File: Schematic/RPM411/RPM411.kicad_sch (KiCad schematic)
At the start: 84 parts, among them J1 02x08_tbd, P1 P_Cap, Q1 tbd (GDS), U1 STM32F100C8Tb8, U2 TS5A9411, U3 TS5A9411, U4 TS5A9411, U5 74LVC3G04, U6 74LVC1G32, U7 TLV70030DDC

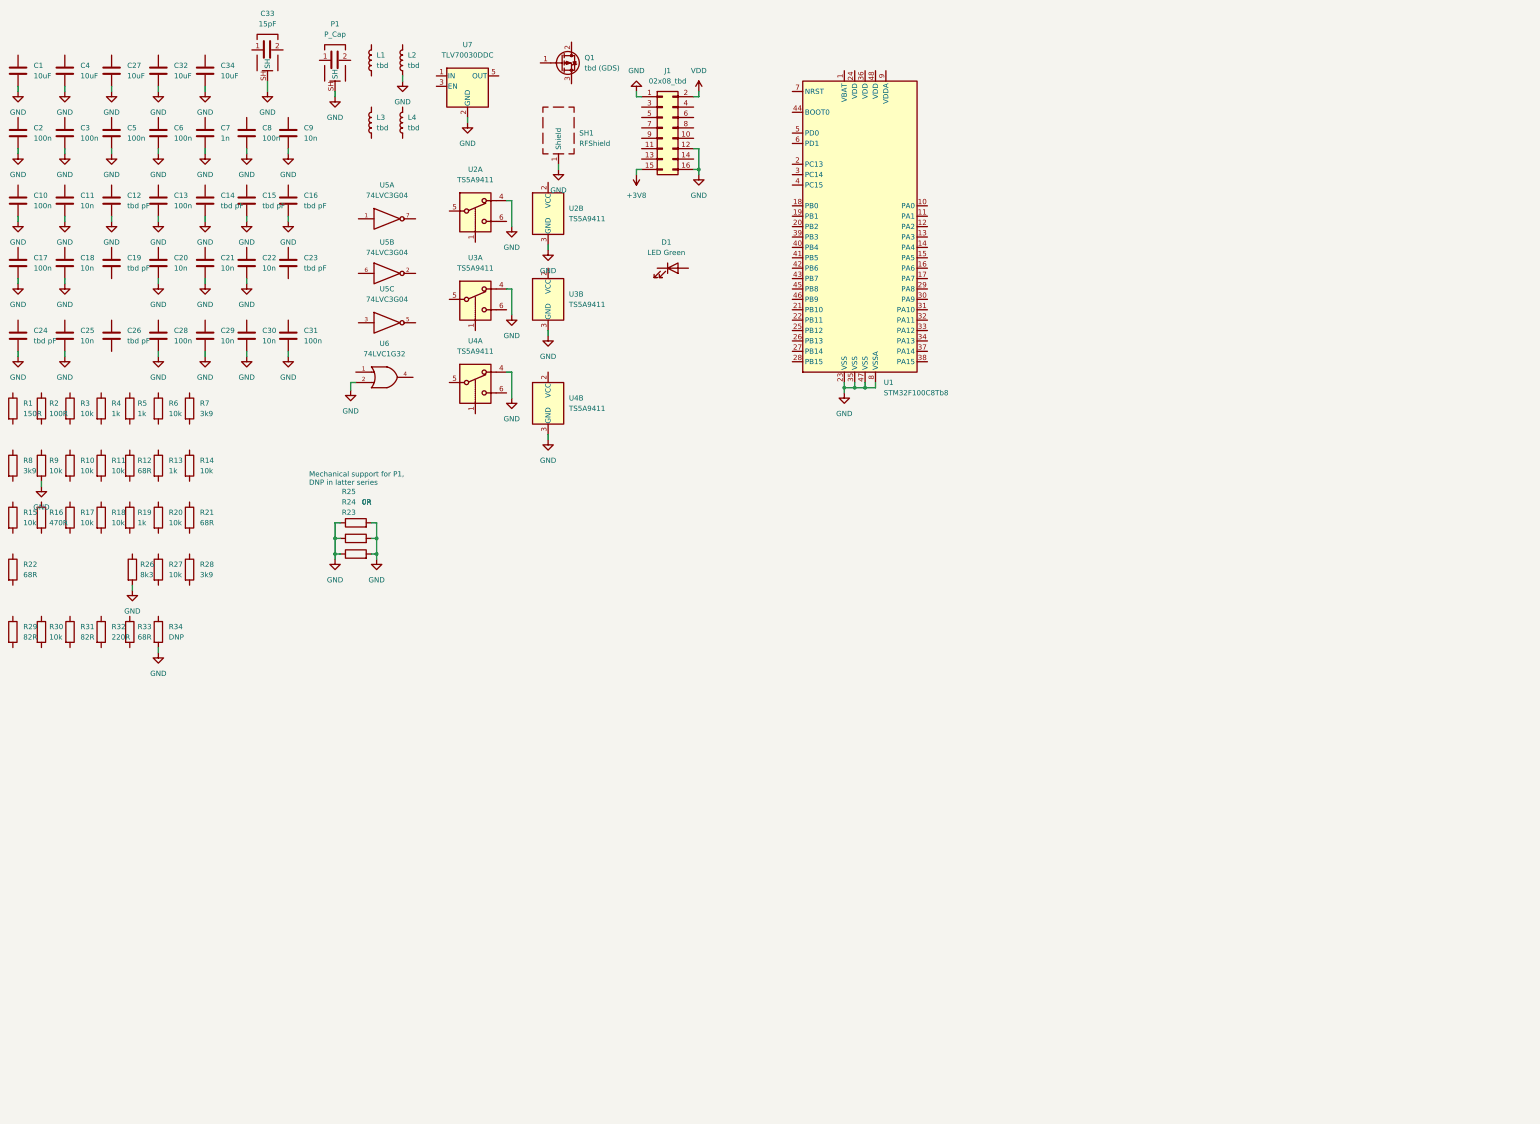
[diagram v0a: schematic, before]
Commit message: completed schematic
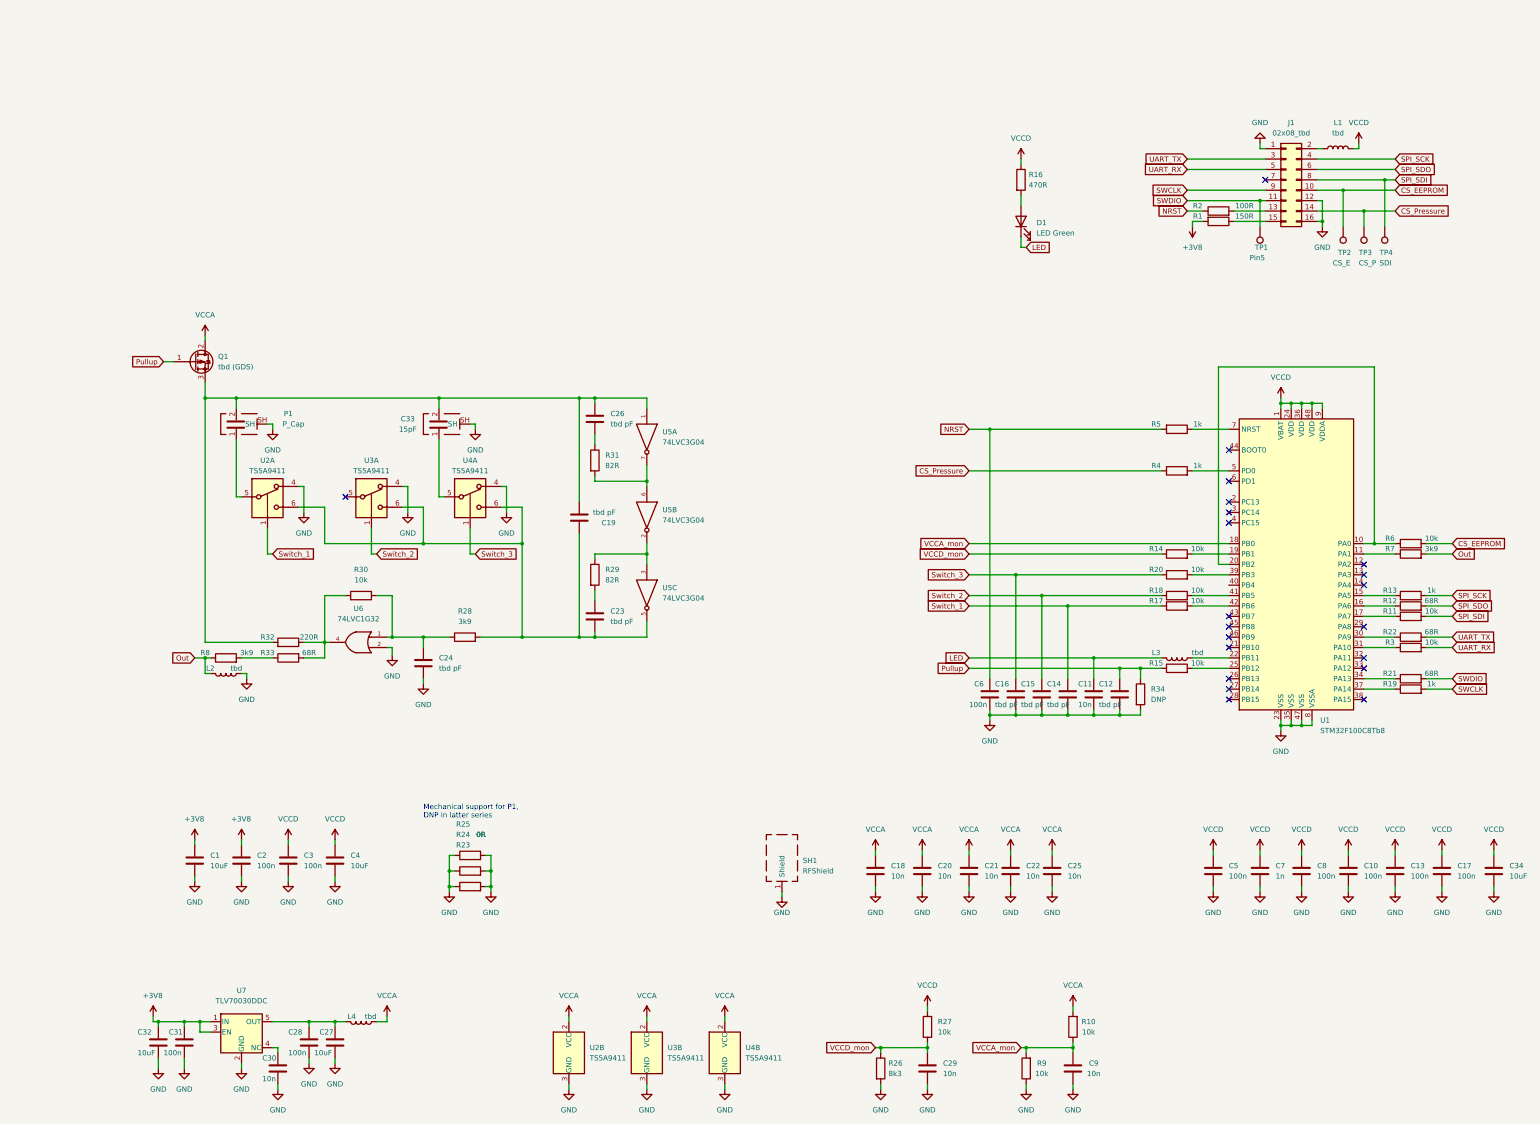
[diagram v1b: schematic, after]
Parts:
- added TP1: Pin5, TestPoint:TestPoint_Pad_D1.0mm, symbol Connector:TestPoint
- added TP2: CS_E, TestPoint:TestPoint_Pad_D1.0mm, symbol Connector:TestPoint
- added TP3: CS_P, TestPoint:TestPoint_Pad_D1.0mm, symbol Connector:TestPoint
- added TP4: SDI, TestPoint:TestPoint_Pad_D1.0mm, symbol Connector:TestPoint
- J1: footprint (none) -> Connector_PinHeader_1.00mm:PinHeader_2x08_P1.00mm_Vertical
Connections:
- net +3V8: now also C1.1, C2.1, C31.1, C32.1, R1.2, U7.1 (IN), U7.3 (EN); no longer J1.15 (Pin_15)
- net GND: now also C12.1, C9.1, R9.1; no longer C12.2, C9.2, R9.2
- net VCC: now also C18.1, C20.1, C21.1, C22.1, C25.1, L4.1, Q1.2 (D), R10.2, U2.2 (VCC), U3.2 (VCC), U4.2 (VCC)
- net VDD: now also C10.1, C13.1, C17.1, C3.1, C34.1, C4.1, C5.1, C7.1, C8.1, L1.2, R16.1, R27.2, U1.1 (VBAT), U1.24 (VDD), U1.36 (VDD), U1.48 (VDD), U1.9 (VDDA); no longer J1.2 (Pin_2)
- net at R29.1: now also U5.2, U5.3
- net at R29.2: now also C23.1
- net Pullup: now reaches Q1.1 (G)
- net Pullup: now also C12.2, R15.1, R34.1
- net at Q1.3 (S): now also C19.1, C26.1, C33.2, P1.2, R32.2, U5.1
- net LED: now reaches C11.1
- net LED: now also D1.1 (K), L3.2
- net at C33.1: now also U4.5
- net VCCA_mon: now reaches R10.1
- net VCCA_mon: now also C9.2, R9.2, U1.18 (PB0)
- net at R12.1: now also U1.16 (PA6)
- net SPI_SDO: now reaches R12.2
- net SPI_SDO: now also J1.6 (Pin_6)
- net at U7.4 (NC): now also C30.1
- net at U7.5 (OUT): now also C27.1, C28.1, L4.2
- net at R22.1: now also U1.30 (PA9)
- net UART_TX: now reaches R22.2
- net UART_TX: now also J1.3 (Pin_3)
- net at U5.6: now also R31.2, U5.7
- net at R13.1: now also U1.15 (PA5)
- net SPI_SCK: now reaches R13.2
- net SPI_SCK: now also J1.4 (Pin_4)
- net at R32.1: now also R30.2, R33.2, U6.4
- net Switch_2: now reaches U3.1
- net Switch_2: now also C15.1, R18.1
- net at U3.6: now also C19.2, C23.2, R28.2, U2.6, U4.6, U5.5
- net at R5.1: now also U1.7 (NRST)
- net NRST: now reaches R5.2
- net NRST: now also C6.1, R2.1
- net at R1.1: now also J1.15 (Pin_15)
- net at R21.1: now also U1.34 (PA13)
- net SWDIO: now reaches R21.2
- net SWDIO: now also J1.11 (Pin_11), TP1.1
- net at R6.1: now also U1.10 (PA0), U1.20 (PB2)
- net CS_EEPROM: now reaches R6.2
- net CS_EEPROM: now also J1.10 (Pin_10), TP2.1
- net at U1.11 (PA1): now also R7.1
- net at U1.17 (PA7): now also R11.1
- net at U1.19 (PB1): now also R14.2
- net at U1.22 (PB11): now also L3.1
- net at U1.25 (PB12): now also R15.2
- net at U1.31 (PA10): now also R3.1
- net at U1.37 (PA14): now also R19.1
- net at U1.39 (PB3): now also R20.2
- net at U1.41 (PB5): now also R18.2
- net at U1.42 (PB6): now also R17.2
- net at U1.5 (PD0): now also R4.2
- net at U6.1: now also C24.1, R28.1, R30.1
- net at D1.2 (A): now also R16.2
- net SWCLK : now reaches R19.2
- net SWCLK : now also J1.9 (Pin_9)
- net Switch_3: now reaches R20.1
- net Switch_3: now also C16.1, U4.1
- net at R33.1: now also R8.2
- net VCCD_mon: now reaches C29.1
- net VCCD_mon: now also R14.1, R26.1, R27.1
- net Out: now reaches R8.1
- net Out: now also L2.2, R7.2
- net at J1.13 (Pin_13): now also R2.2
- net CS_Pressure: now reaches J1.14 (Pin_14)
- net CS_Pressure: now also R4.1, TP3.1
- net UART_RX: now reaches J1.5 (Pin_5)
- net UART_RX: now also R3.2
- net SPI_SDI: now reaches J1.8 (Pin_8)
- net SPI_SDI: now also R11.2, TP4.1
- net at C26.2: now also R31.1
- net Switch_1: now reaches R17.1
- net Switch_1: now also C14.1, U2.1
- net at P1.1: now also U2.5
- net at L1.1: now also J1.2 (Pin_2)
- no-connect marks 0 -> 21
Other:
- moved on the sheet: C1, C10, C11, C12, C13, C14, C15, C16, C17, C18, C19, C2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
